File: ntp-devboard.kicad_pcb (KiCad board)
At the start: 2 copper layers, 42.4 x 51 mm, 74 parts, among them J1 USB_C_Receptacle_USB2.0_14P, J2 Conn_01x07, J3 Conn_01x20, J4 Conn_01x04, J5 Conn_01x02, J6 RJ45_Hanrun_HR911105A_Horizon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, SW1 SW_Push, U1 RP2040, U2 MCP1700x-330xxTT, U3 LAN9250/ML, U4 W25Q16JVUXIQ TR, Y1 12 MHz, Y2 25 MHz

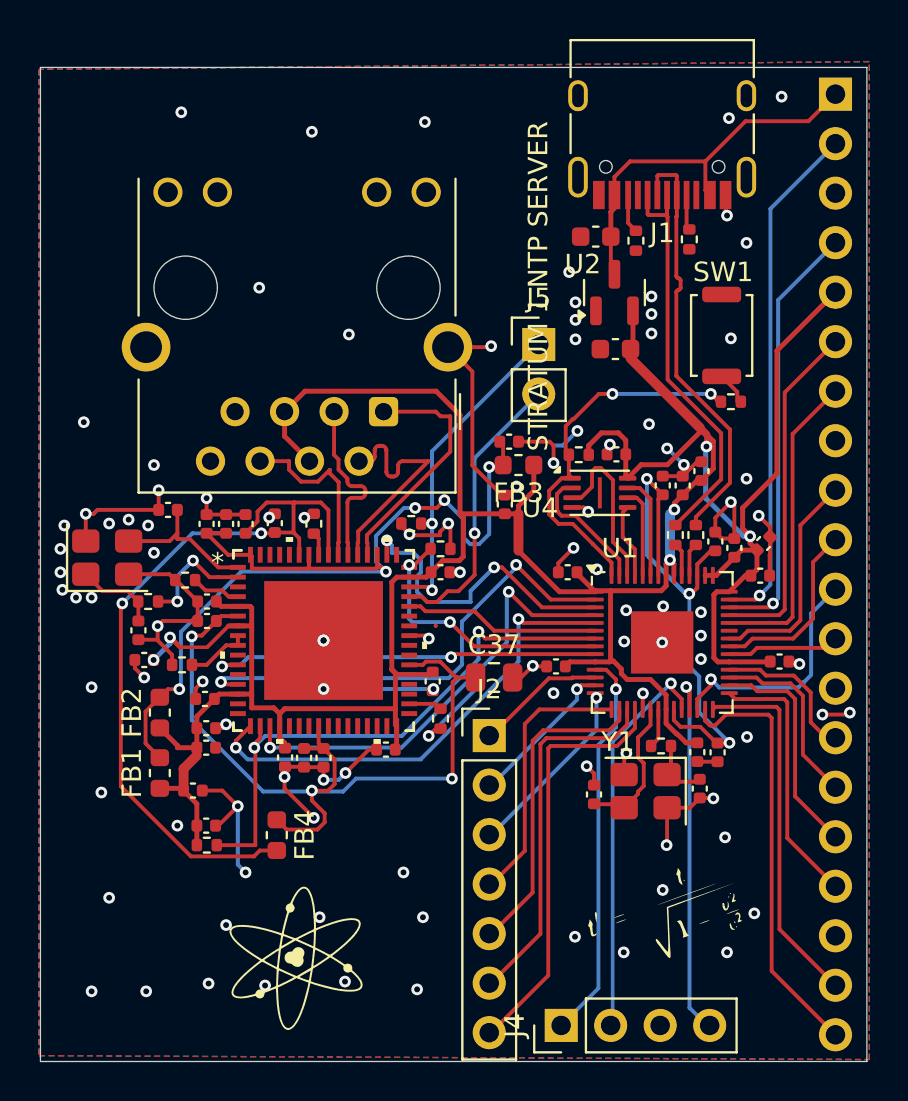
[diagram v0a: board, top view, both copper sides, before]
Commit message: update sch and pcb
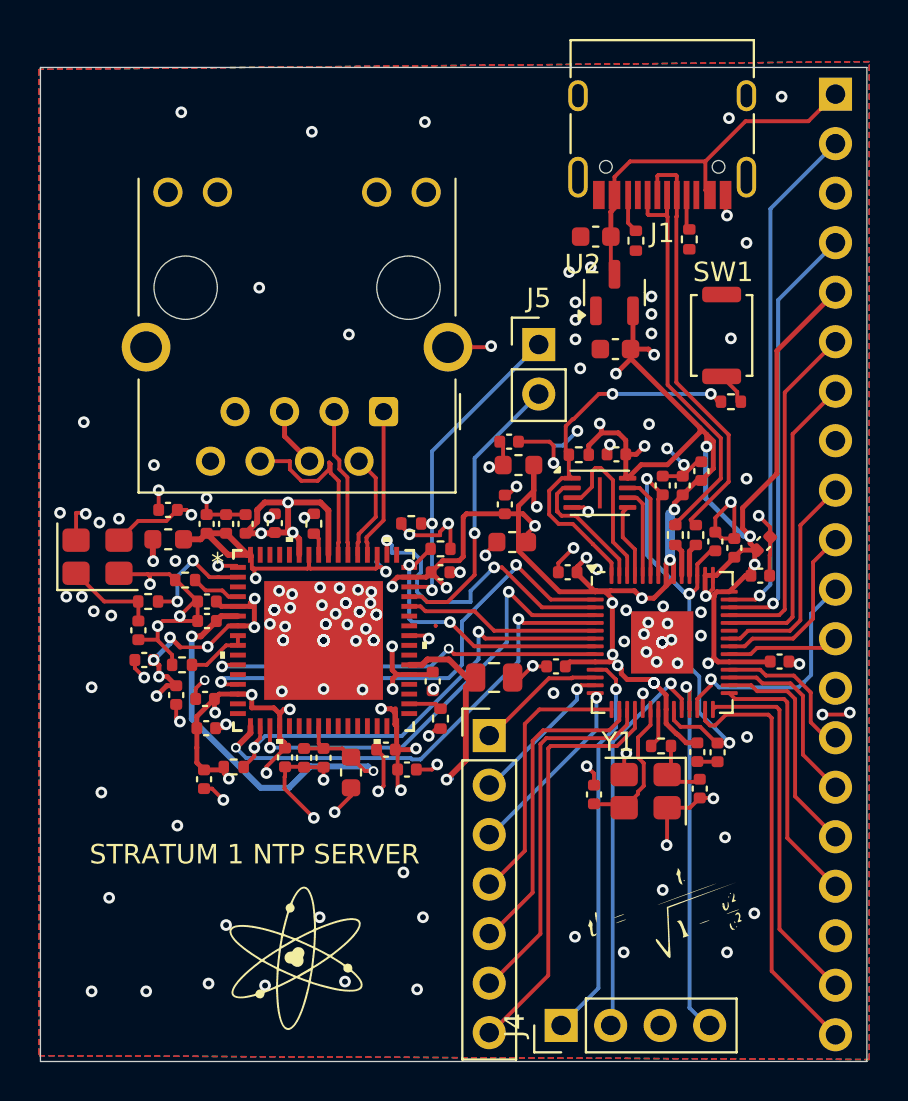
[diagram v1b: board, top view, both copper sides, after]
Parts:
- moved FB1 21.6 mm to (145.7, 106.5), turned to 180 degrees
- moved C21 11.0 mm to (140.3, 118.1)
- moved FB2 8.90 mm to (128.0, 106.3), turned to 0 degrees
- moved FB4 4.99 mm to (137.4, 118.3)
- moved R11 4.24 mm to (131.4, 118.0)
- moved C31 3.11 mm to (128.4, 114.3), turned to -90 degrees
- moved C20 2.38 mm to (129.9, 118.6), turned to 90 degrees
- moved Y2 0.50 mm to (124.4, 107.2)
- turned R13 to 0 degrees
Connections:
- net C34 renamed Power_Lan
- net C35 renamed POWER_LAN12
- net C40 renamed TXRX_POWER
- R13 pad 1: Net-(U3-FXLOSEN) -> GND
- R13 pad 2: GND -> Net-(U3-FXLOSEN)
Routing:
- net TXRX_POWER: track 48.8 -> 35.3 mm, vias 5 -> 4
- net GND: track 102.4 -> 90.0 mm, vias 105 -> 233
- net POWER_LAN12: track 39.8 -> 30.6 mm, vias 2 -> 4
- net TX+: track 12.3 -> 5.92 mm
- net +3V3: track 166.1 -> 159.7 mm, vias 6 -> 40
- net GPIO5: track 29.3 -> 23.4 mm
- net TX-: track 12.4 -> 7.73 mm
- net Power_Lan: track 42.3 -> 38.4 mm
- net RX-: track 9.04 -> 7.64 mm
- net OSIN: track 7.67 -> 8.70 mm, vias 0 -> 2
- net RX+: track 9.08 -> 9.76 mm
- net Net-(C19-Pad2): track 4.27 -> 4.78 mm
- net (no net): vias 0 -> 5
- added copper zone on In2.Cu, net +3V3
- added copper zone on In1.Cu, net GND
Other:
- copper layers 2 -> 4
